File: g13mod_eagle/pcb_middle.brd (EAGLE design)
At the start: 134.2 x 33.2 mm, 80 parts

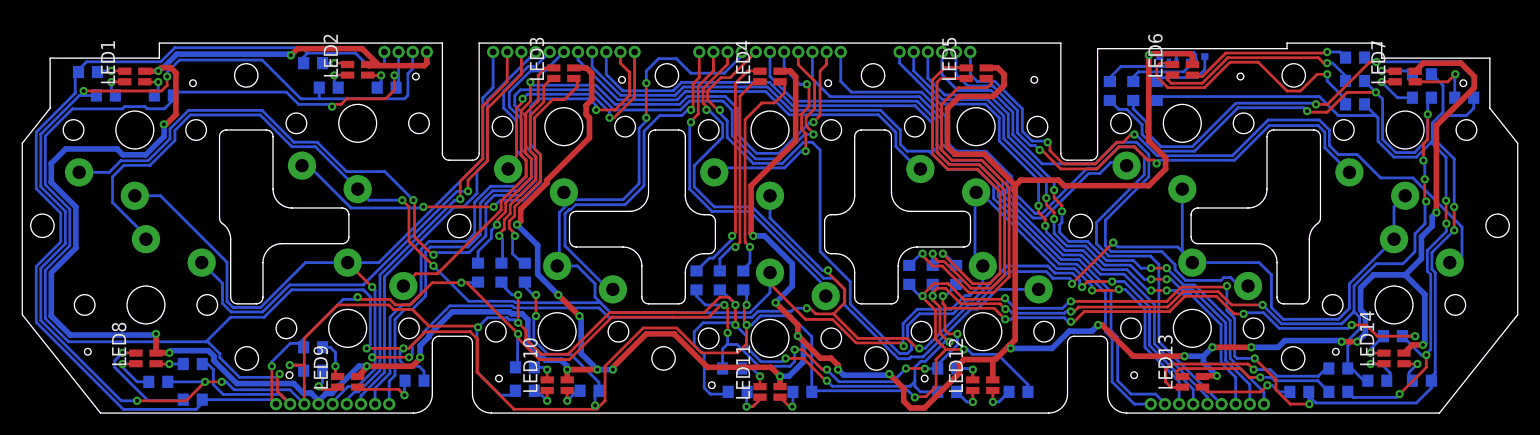
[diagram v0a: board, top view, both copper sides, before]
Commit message: Fix bug
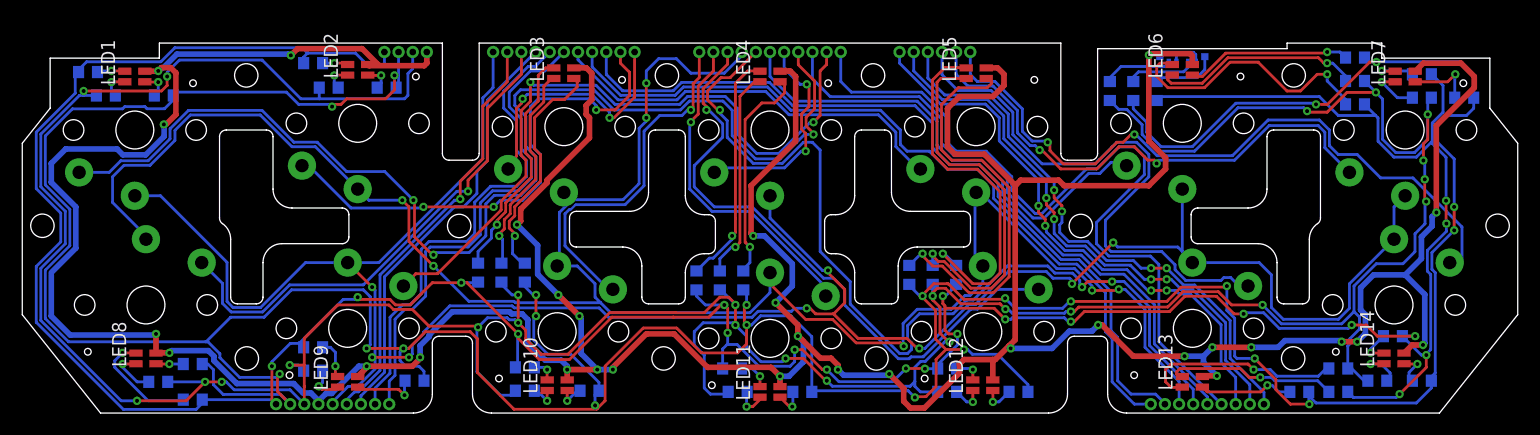
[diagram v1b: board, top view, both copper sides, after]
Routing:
- net V: track 409.6 -> 404.0 mm
- net CN6_18: track 205.8 -> 204.7 mm
- net CN7_15: track 186.3 -> 185.5 mm
- net G: track 326.6 -> 326.0 mm
- net N$20: track 4.59 -> 4.08 mm
- net N$39: track 9.02 -> 8.52 mm
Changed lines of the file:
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@@
 <wire x1="-50.9" y1="-24.47255" x2="-50.9" y2="-24.2" width="0.254" layer="16"/>
 <contactref element="R26" pad="1"/>
-<wire x1="-41.85" y1="-19.5" x2="-41.7" y2="-19.5" width="0.254" layer="16"/>
 <wire x1="-43.05" y1="-19.15" x2="-44.7" y2="-20.8" width="0.254" layer="16"/>
 <wire x1="-44.7" y1="-21.2" x2="-44.7" y2="-20.8" width="0.254" layer="16"/>
@@
 <wire x1="-34.6" y1="6.995" x2="-34.605" y2="7" width="0.254" layer="16"/>
 <wire x1="-37.2" y1="6.9" x2="-36" y2="5.7" width="0.254" layer="16"/>
-<wire x1="-41.7" y1="6.15" x2="-41.85" y2="6" width="0.254" layer="16"/>
 <wire x1="-41.85" y1="6" x2="-41.875" y2="6.025" width="0.254" layer="16"/>
 <wire x1="-41.875" y1="6.025" x2="-41.875" y2="6.525" width="0.254" layer="16"/>
@@
 <via x="-33.7" y="4.9" extent="1-16" drill="0.35"/>
 <contactref element="R27" pad="1"/>
-<wire x1="-43.06" y1="-24.56" x2="-43.06" y2="-24.6" width="0.254" layer="1"/>
 <via x="-32.9" y="-19.6" extent="1-16" drill="0.35"/>
 <wire x1="-32.9" y1="-19.6" x2="-33.2" y2="-19.9" width="0.254" layer="16"/>
@@
 <wire x1="-35.873" y1="-19.273" x2="-36.2" y2="-19.6" width="0.254" layer="16"/>
 <wire x1="-35.873" y1="-14.9603875" x2="-35.873" y2="-19.273" width="0.254" layer="16"/>
-<wire x1="-33.435" y1="4.9" x2="-33.7" y2="4.9" width="0.254" layer="16"/>
 <contactref element="R30" pad="1"/>
 <wire x1="-21.25" y1="-14.8" x2="-22" y2="-14.05" width="0.254" layer="16"/>
@@
 <wire x1="-56.8" y1="-24.3" x2="-52.4" y2="-24.3" width="0.254" layer="1"/>
 <wire x1="-52.4" y1="-24.3" x2="-50.7" y2="-22.6" width="0.254" layer="1"/>
-<wire x1="-60.75" y1="2.8" x2="-60.45" y2="3.1" width="0.254" layer="16"/>
 <via x="-61.6" y="3.5" extent="1-16" drill="0.35"/>
 <wire x1="-54.6" y1="3.5" x2="-61.6" y2="3.5" width="0.254" layer="1"/>
@@
 <wire x1="53.3" y1="-22.5" x2="53.65" y2="-22.5" width="0.254" layer="16"/>
 <wire x1="52.2" y1="-21.4" x2="53.3" y2="-22.5" width="0.254" layer="16"/>
-<wire x1="51.85" y1="-21.4" x2="52" y2="-21.25" width="0.254" layer="16"/>
 <wire x1="52.4064" y1="-16.2936" x2="52.4064" y2="-14" width="0.254" layer="16"/>
 <wire x1="52.4064" y1="-14" x2="54.4064" y2="-12" width="0.254" layer="16"/>
@@
 <via x="-22.7" y="-8.5" extent="1-16" drill="0.35"/>
 <via x="-19" y="-14.8" extent="1-16" drill="0.35"/>
-<wire x1="-18.2" y1="-21.2" x2="-18.7936" y2="-20.6064" width="0.254" layer="16"/>
-<wire x1="-18.7936" y1="-20.6064" x2="-20.03495" y2="-20.6064" width="0.254" layer="16"/>
 <wire x1="-55.1" y1="-20" x2="-55.1" y2="-20.025" width="0.254" layer="1"/>
 <via x="-55.1" y="-18.3" extent="1-16" drill="0.35"/>
 <via x="-54.4" y="0.5" extent="1-16" drill="0.35"/>
-<wire x1="-37" y1="-22.125" x2="-36.725" y2="-22.125" width="0.254" layer="1"/>
 <wire x1="-64.5" y1="-12.8" x2="-64.5" y2="-13" width="0.254" layer="16"/>
 <via x="0.9" y="-22.1" extent="1-16" drill="0.35"/>
@@
 <via x="-1.5" y="-9.5" extent="1-16" drill="0.35"/>
 <via x="-15.5" y="-21.5" extent="1-16" drill="0.35"/>
-<wire x1="-17" y1="-16.8" x2="-17.1" y2="-16.7" width="0.254" layer="16"/>
-<wire x1="-17" y1="-16.8" x2="-17" y2="-18" width="0.254" layer="16"/>
 <via x="-17.1" y="-16.7" extent="1-16" drill="0.35"/>
 <via x="-14.1" y="-21.5" extent="1-16" drill="0.35"/>
-<wire x1="19.4" y1="5.575" x2="19.525" y2="5.7" width="0.254" layer="1"/>
 <wire x1="21.7625" y1="-19.0625" x2="21.8686" y2="-18.9564" width="0.254" layer="1"/>
 <wire x1="21.4125" y1="-19.4125" x2="20" y2="-20.825" width="0.254" layer="1"/>
 <via x="6.1" y="-21.5" extent="1-16" drill="0.35"/>
 <via x="10.7" y="-21.9" extent="1-16" drill="0.35"/>
-<wire x1="36.47" y1="6" x2="36.5" y2="6.03" width="0.2032" layer="16"/>
 <via x="34" y="6.72125" extent="1-16" drill="0.35"/>
 <wire x1="36.5" y1="6.97245" x2="38" y2="6.97245" width="0.254" layer="16"/>
@@
 <via x="59.8" y="-7.4" extent="1-16" drill="0.35"/>
 <wire x1="37.9" y1="6" x2="37.9" y2="5.875" width="0.254" layer="1"/>
-<wire x1="37.7875" y1="6.7875" x2="37.60255" y2="6.97245" width="0.254" layer="1"/>
-<wire x1="37" y1="6.97245" x2="37.60255" y2="6.97245" width="0.254" layer="1"/>
-<wire x1="34.9975" y1="6.8025" x2="34.82755" y2="6.97245" width="0.254" layer="16"/>
 <wire x1="34.2512" y1="6.97245" x2="34" y2="6.72125" width="0.254" layer="16"/>
 <wire x1="34.2512" y1="6.97245" x2="34.82755" y2="6.97245" width="0.254" layer="16"/>
@@
 <wire x1="21.8686" y1="-18.9564" x2="22" y2="-18.825" width="0.508" layer="1"/>
 <wire x1="22" y1="-18.825" x2="22" y2="-5.3956" width="0.508" layer="1"/>
-<wire x1="22" y1="-5.3956" x2="22" y2="-4.8686" width="0.508" layer="1"/>
 <wire x1="19.4" y1="5.575" x2="20.425" y2="5.575" width="0.508" layer="1"/>
 <wire x1="20.425" y1="5.575" x2="21" y2="5" width="0.508" layer="1"/>
@@
 <via x="-32.4" y="-20.4" extent="1-16" drill="0.35"/>
 <via x="-35.7" y="-20.4" extent="1-16" drill="0.35"/>
-<wire x1="-37.9" y1="-11.9" x2="-36.8" y2="-11.9" width="0.254" layer="16"/>
 <via x="-35.7" y="-14.1" extent="1-16" drill="0.35"/>
 <wire x1="-35.7" y1="-14.1" x2="-37.9" y2="-11.9" width="0.254" layer="1"/>
@@
 <wire x1="-30.9" y1="-14.9" x2="-30.9" y2="-10.9" width="0.254" layer="16"/>
 <wire x1="-21.4064" y1="-2.5936" x2="-22.3128" y2="-1.6872" width="0.254" layer="16"/>
-<wire x1="-21.4064" y1="-4.3316625" x2="-21.4064" y2="-4.3064" width="0.254" layer="16"/>
 <wire x1="-21.4064" y1="-4.3064" x2="-21.4064" y2="-2.5936" width="0.254" layer="16"/>
 <wire x1="-34.17" y1="-24.6" x2="-34.17" y2="-22.5400125" width="0.254" layer="16"/>
@@
 <wire x1="-14.8" y1="-14" x2="-18.4" y2="-10.4" width="0.254" layer="16"/>
 <wire x1="-18.4" y1="-10.4" x2="-18.4" y2="-7.5254" width="0.254" layer="16"/>
-<wire x1="-18.024" y1="-7.124" x2="-17.9986" y2="-7.124" width="0.2032" layer="16"/>
 <wire x1="-17.8687375" y1="-7.124" x2="-17.4447375" y2="-6.7" width="0.2032" layer="16"/>
 <wire x1="-9.9" y1="1.3" x2="-7.9" y2="1.3" width="0.254" layer="16"/>
@@
 <contactref element="JP3" pad="10"/>
 <contactref element="G11" pad="CHOC2"/>
-<wire x1="-5.08" y1="7" x2="-5.08" y2="6.92" width="0.254" layer="1"/>
 <via x="-7.1" y="0.7" extent="1-16" drill="0.35"/>
 <wire x1="5" y1="-14.1" x2="5" y2="-14.9" width="0.254" layer="16"/>
@@
 <via x="28.9" y="-14.4" extent="1-16" drill="0.35"/>
 <wire x1="28.9" y1="-14" x2="28.9" y2="-14.4" width="0.254" layer="16"/>
-<wire x1="19" y1="-12.2" x2="19.1" y2="-12.2" width="0.254" layer="16"/>
 <via x="12" y="-19.4" extent="1-16" drill="0.35"/>
 <wire x1="36.71" y1="-24.6" x2="36.71" y2="-22.559475" width="0.254" layer="16"/>
@@
 <wire x1="18.5" y1="-6.5" x2="18.4" y2="-6.6" width="0.254" layer="16"/>
 <wire x1="18.4" y1="-6.6" x2="18.4" y2="-11.5" width="0.254" layer="16"/>
-<wire x1="19" y1="-12.2" x2="18.5" y2="-11.7" width="0.254" layer="16"/>
 <wire x1="-19.1" y1="-12.2" x2="-18.9" y2="-12" width="0.254" layer="16"/>
 <wire x1="-18.9" y1="-12" x2="-18.9" y2="-7.4" width="0.254" layer="16"/>
@@
 <contactref element="R16" pad="2"/>
 <contactref element="LED6" pad="1"/>
-<wire x1="51.65" y1="4.4" x2="51.6" y2="4.4" width="0.2032" layer="16"/>
 <via x="50" y="6" extent="1-16" drill="0.35"/>
 <wire x1="51.65" y1="4.4" x2="51.65" y2="4.85" width="0.254" layer="16"/>
@@
 <contactref element="R20" pad="2"/>
 <contactref element="LED7" pad="2"/>
-<wire x1="57.65" y1="5" x2="57.6" y2="5" width="0.2032" layer="16"/>
-<wire x1="57.6" y1="5" x2="57.3" y2="5.3" width="0.2032" layer="16"/>
 <via x="54.9" y="5.3" extent="1-16" drill="0.35"/>
-<wire x1="56.075" y1="5.3" x2="56.1" y2="5.275" width="0.2032" layer="1"/>
 <wire x1="56.1" y1="5.275" x2="54.925" y2="5.275" width="0.254" layer="1"/>
 <wire x1="54.925" y1="5.275" x2="54.9" y2="5.3" width="0.254" layer="1"/>
@@
 <contactref element="R27" pad="2"/>
 <contactref element="LED9" pad="4"/>
-<wire x1="-33" y1="-22.75" x2="-32.75" y2="-22.5" width="0.254" layer="16"/>
 <wire x1="-32.8" y1="-23.8" x2="-33.325" y2="-23.275" width="0.254" layer="1"/>
 <wire x1="-33.325" y1="-23.275" x2="-36.8" y2="-23.275" width="0.254" layer="1"/>
@@
 <contactref element="LED13" pad="4"/>
 <via x="44.6387875" y="-22.9088" extent="1-16" drill="0.35"/>
-<wire x1="38.8" y1="-23.075" x2="39.3" y2="-23.075" width="0.2032" layer="1"/>
 <wire x1="46.65" y1="-23.5" x2="45.65" y2="-23.5" width="0.254" layer="16"/>
 <wire x1="45.65" y1="-23.5" x2="45.0588" y2="-22.9088" width="0.254" layer="16"/>
